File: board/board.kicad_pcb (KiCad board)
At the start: 2 copper layers, 53 x 42 mm, 35 parts, among them J1 ANT, J2 DEBUG, J3 GPIO, P1 USB_C_Plug_USB2.0, SW1 BOOTSEL, SW2 RUN, U1 RP2040, U2 W25Q128JVS, U3 NCP1117-3.3_SOT223, U4 RFM95W-915S2, Y1 ABM8G-12.000MHZ-18-D2Y-T

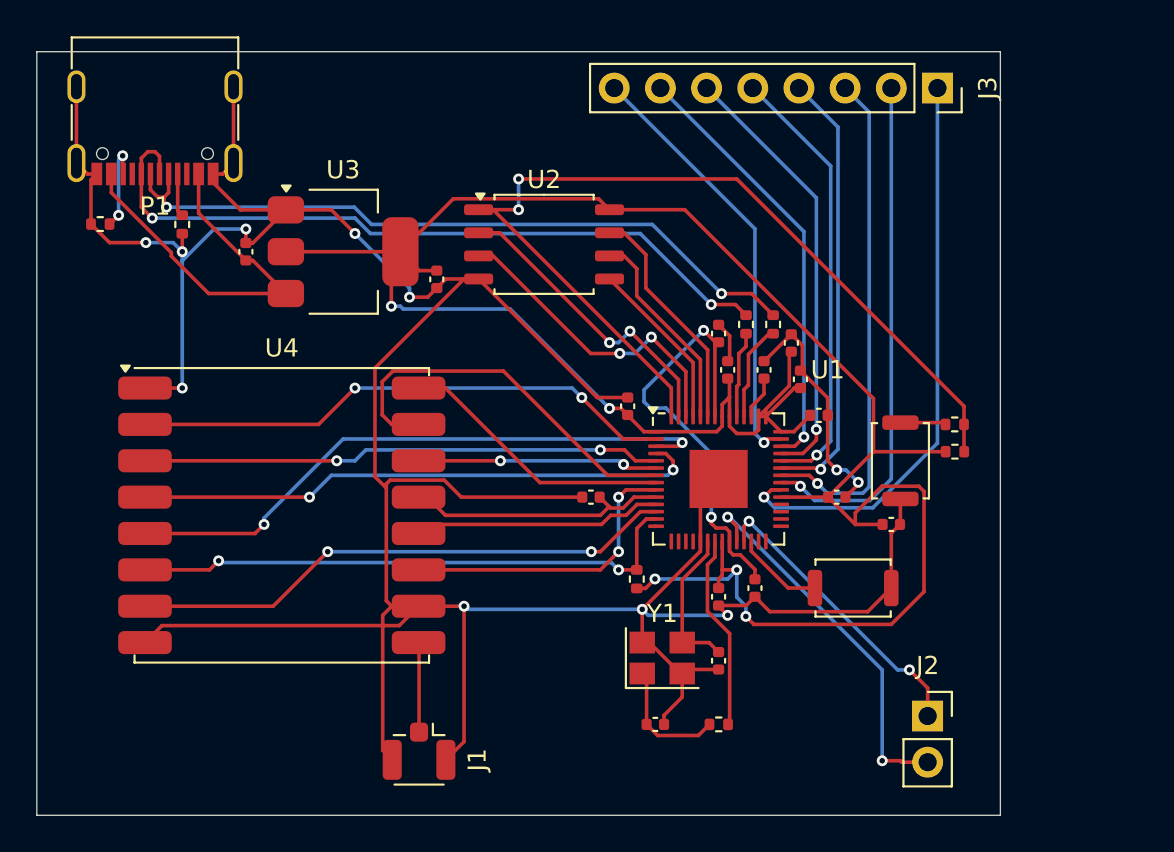
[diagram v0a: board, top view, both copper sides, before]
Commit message: board v2 hour 1
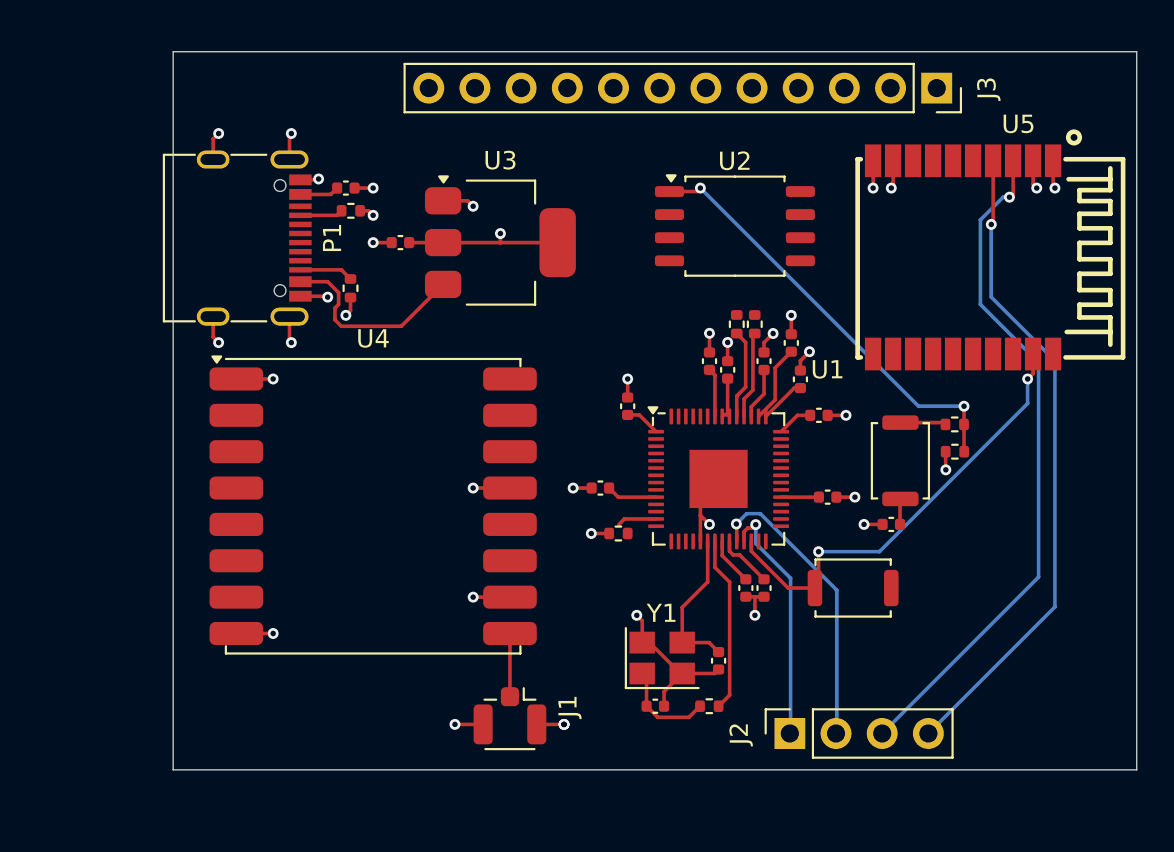
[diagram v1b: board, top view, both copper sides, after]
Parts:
- added U5: BLE5201, BLE5201:BLE5201, F.Cu at (85.5, 37.8)
- J2: footprint Connector_PinSocket_2.54mm:PinSocket_1x02_P2.54mm_Vertical -> Connector_PinSocket_2.54mm:PinSocket_1x04_P2.54mm_Vertical
- J3: footprint Connector_PinSocket_2.54mm:PinSocket_1x08_P2.54mm_Vertical -> Connector_PinSocket_2.54mm:PinSocket_1x12_P2.54mm_Vertical
- moved R4 14.2 mm to (51.8, 39.5), turned to -90 degrees
- moved U2 10.5 mm to (72.9, 36.1)
- moved R3 9.31 mm to (51.8, 35.2), turned to 0 degrees
- moved U3 8.66 mm to (60.0, 37.0)
- moved P1 8.42 mm to (45.3, 36.8), turned to -90 degrees
- moved J2 7.64 mm to (75.9, 64.0), turned to 90 degrees
- moved C12 6.52 mm to (51.5, 34.0), turned to 0 degrees
- moved J1 5.37 mm to (60.5, 63.0)
- moved U4 5.05 mm to (53.0, 51.5)
- moved C13 2.84 mm to (54.5, 37.0), turned to 180 degrees
- moved R8 2.71 mm to (66.5, 53.0), turned to 0 degrees
- moved C10 1.60 mm to (71.5, 43.5)
- moved C3 1.57 mm to (73.5, 56.0)
- moved R7 1.13 mm to (71.5, 62.5)
- moved R1 1.01 mm to (74.0, 41.5)
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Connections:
- net Net-(U1-RUN) renamed /RUN
- U1 pad 14: unconnected-(U1-GPIO11-Pad14) -> Net-(U1-GPIO11)
- U1 pad 15: unconnected-(U1-GPIO12-Pad15) -> Net-(U1-GPIO12)
- U1 pad 16: unconnected-(U1-GPIO13-Pad16) -> Net-(U1-GPIO13)
- U1 pad 17: unconnected-(U1-GPIO14-Pad17) -> Net-(U1-GPIO14)
- U1 pad 18: unconnected-(U1-GPIO15-Pad18) -> /PB00
- U1 pad 27: unconnected-(U1-GPIO16-Pad27) -> /PB01
- U1 pad 28: unconnected-(U1-GPIO17-Pad28) -> /PB02
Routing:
- net GND: track 203.4 -> 52.9 mm, vias 11 -> 31
- net +3V3: track 147.2 -> 37.5 mm, vias 5 -> 7
- net Net-(P1-D+-PadA6): track 40.6 -> 0.00 mm, vias 2 -> 0
- net Net-(P1-D--PadA7): track 39.6 -> 0.00 mm, vias 2 -> 0
- net /BLE_SWCLK: track 0.00 -> 37.3 mm, vias 0 -> 1
- net /BLE_SWDIO: track 0.00 -> 35.9 mm, vias 0 -> 1
- net Net-(U1-GPIO1): track 33.5 -> 0.00 mm, vias 2 -> 0
- net Net-(J3-Pin_1): track 31.9 -> 0.00 mm, vias 1 -> 0
- net Net-(U1-GPIO2): track 31.3 -> 0.00 mm, vias 2 -> 0
- net /DIO5: track 30.3 -> 0.00 mm, vias 2 -> 0
- net Net-(U1-GPIO0): track 30.1 -> 0.00 mm, vias 2 -> 0
- net Net-(U1-GPIO10): track 31.0 -> 2.17 mm, vias 2 -> 0
- net Net-(U1-GPIO3): track 28.6 -> 0.00 mm, vias 2 -> 0
- net Net-(U1-QSPI_SS): track 52.3 -> 23.8 mm
- net Net-(J3-Pin_2): track 28.5 -> 0.00 mm, vias 1 -> 0
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- added copper zone on In2.Cu, net +3V3
- added copper zone on In1.Cu, net GND
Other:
- board size 53 x 42 mm -> 53 x 39.5 mm
- copper layers 2 -> 4
- board text removed: "YARLo design by scarlettekk v1"
